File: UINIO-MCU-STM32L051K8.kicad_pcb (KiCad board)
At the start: 2 copper layers, 48.4 x 20.5 mm, 33 parts, among them J1 Conn_01x14_Male, J2 Conn_01x14_Male, J3 Conn_01x04_Male, SW1 SW_Push, SW2 SW_Push, U1 ME6211, U2 W25Q128JVSSIQ, U3 STM32L051K8U6, Y1 Crystal-FC135-32.768

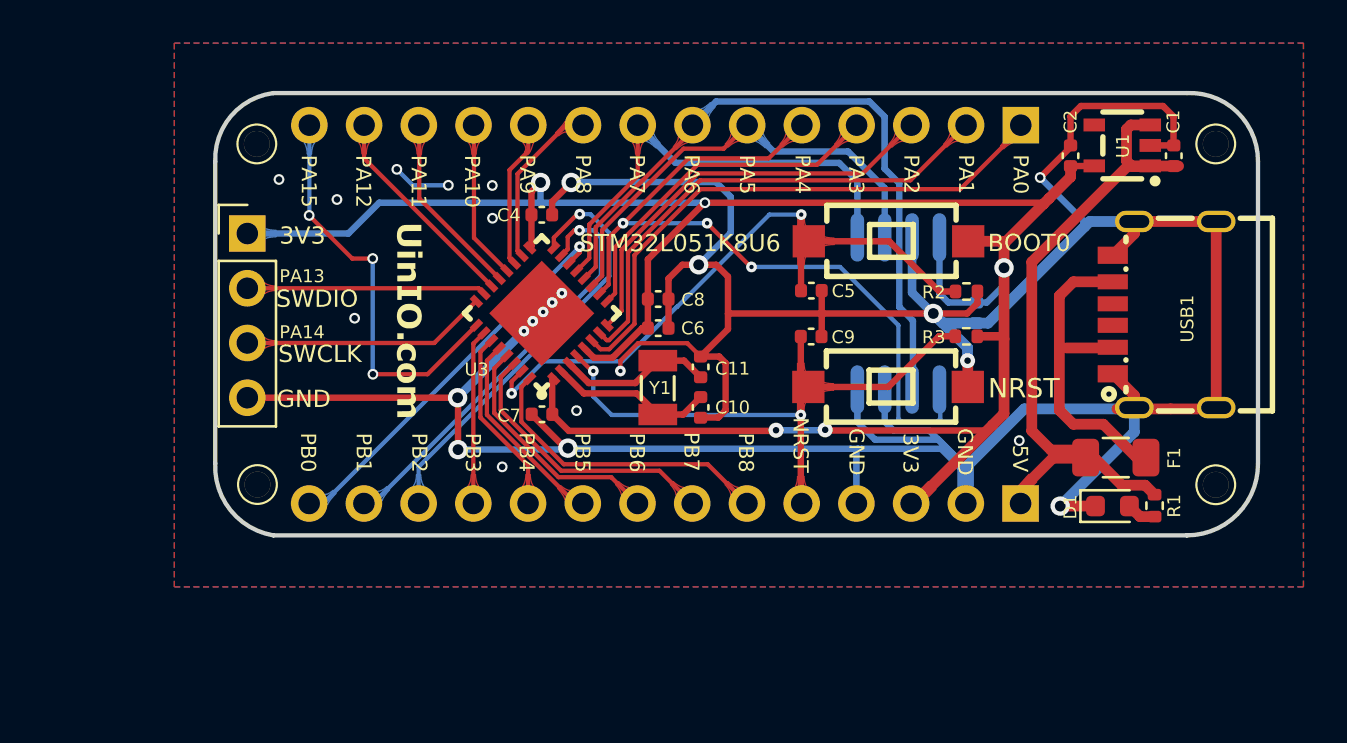
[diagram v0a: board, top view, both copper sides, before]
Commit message: Release UINIO-MCU-STM32L051K8 version 3.2.0.
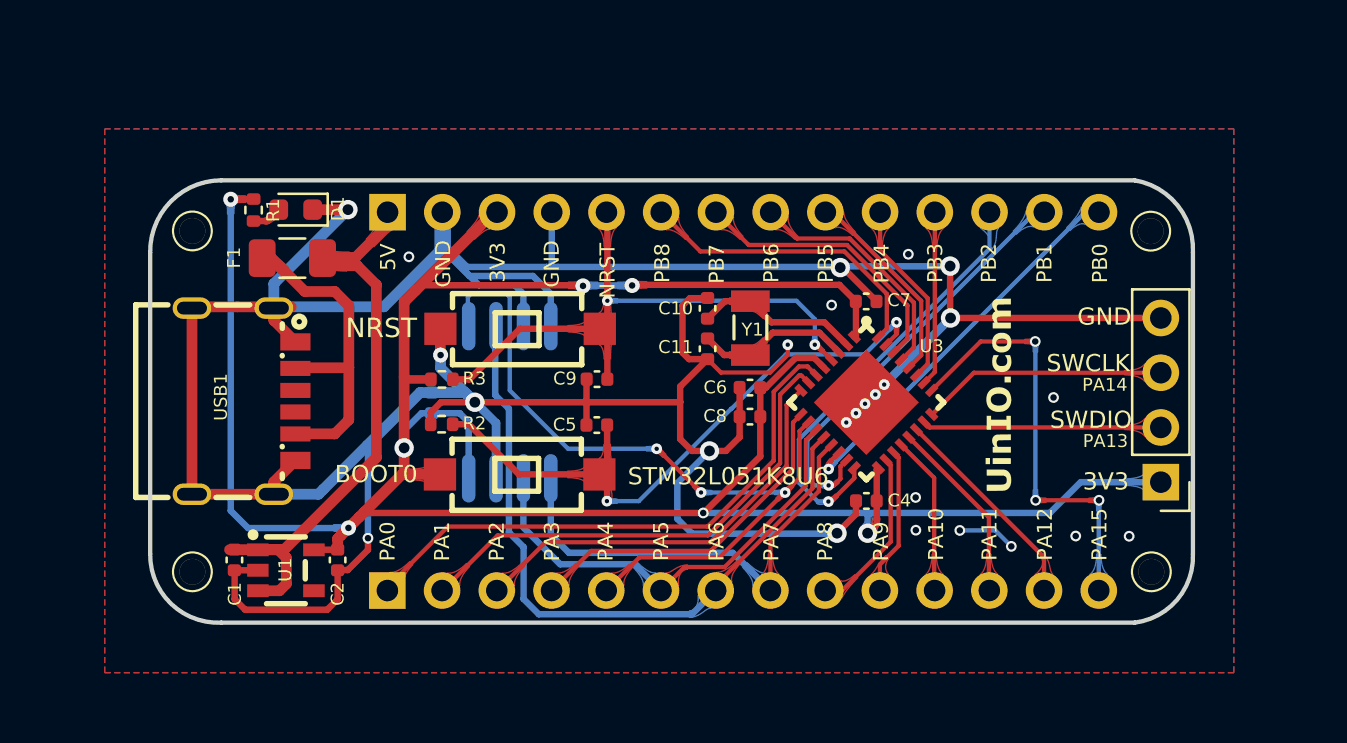
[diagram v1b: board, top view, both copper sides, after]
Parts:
- moved Hole4 51.5 mm to (127.5, 111.7), turned to 180 degrees
- moved Hole3 48.9 mm to (127.5, 95.8), turned to 180 degrees
- moved C1 47.5 mm to (129.5, 111.1), turned to 90 degrees
- moved Hole1 46.0 mm to (172.1, 111.7), turned to 180 degrees
- moved R1 44.0 mm to (130.4, 94.9)
- moved J3 43.9 mm to (172.5, 107.5), turned to 180 degrees
- moved U1 43.5 mm to (131.9, 111.6), turned to 180 degrees
- moved Hole2 43.1 mm to (172.0, 95.9), turned to 180 degrees
- moved USB1 42.9 mm to (129.9, 103.8), turned to -90 degrees
- moved D1 40.3 mm to (132.3, 94.9), turned to 180 degrees
- moved F1 39.3 mm to (132.2, 97.1), turned to 0 degrees
- moved C2 38.8 mm to (134.3, 111.1), turned to 90 degrees
- moved J1 36.5 mm to (136.6, 112.5), turned to -90 degrees
- moved J2 32.3 mm to (136.6, 95.0), turned to -90 degrees
- moved ? 32.0 mm to (135.4, 103.7), turned to -90 degrees
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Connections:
- R1 pad 2: /VDD_5V -> /VDD_3.3V
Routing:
- net /VDD_3.3V: track 104.8 -> 126.1 mm, vias 5 -> 7
- net /VDD_5V: track 31.5 -> 28.0 mm
- net GND: track 186.5 -> 188.0 mm
- net /PA15: track 19.1 -> 20.3 mm
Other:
- outline, holes or cut-outs redrawn
- board text added: "Version 3.2.0"
- board text removed: "Version 3.1.0"

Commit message: Update version.
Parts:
- J1, J2: value Conn_01x14_Male -> Conn_01x14_Pin
- J3: value Conn_01x04_Male -> Conn_01x04_Pin

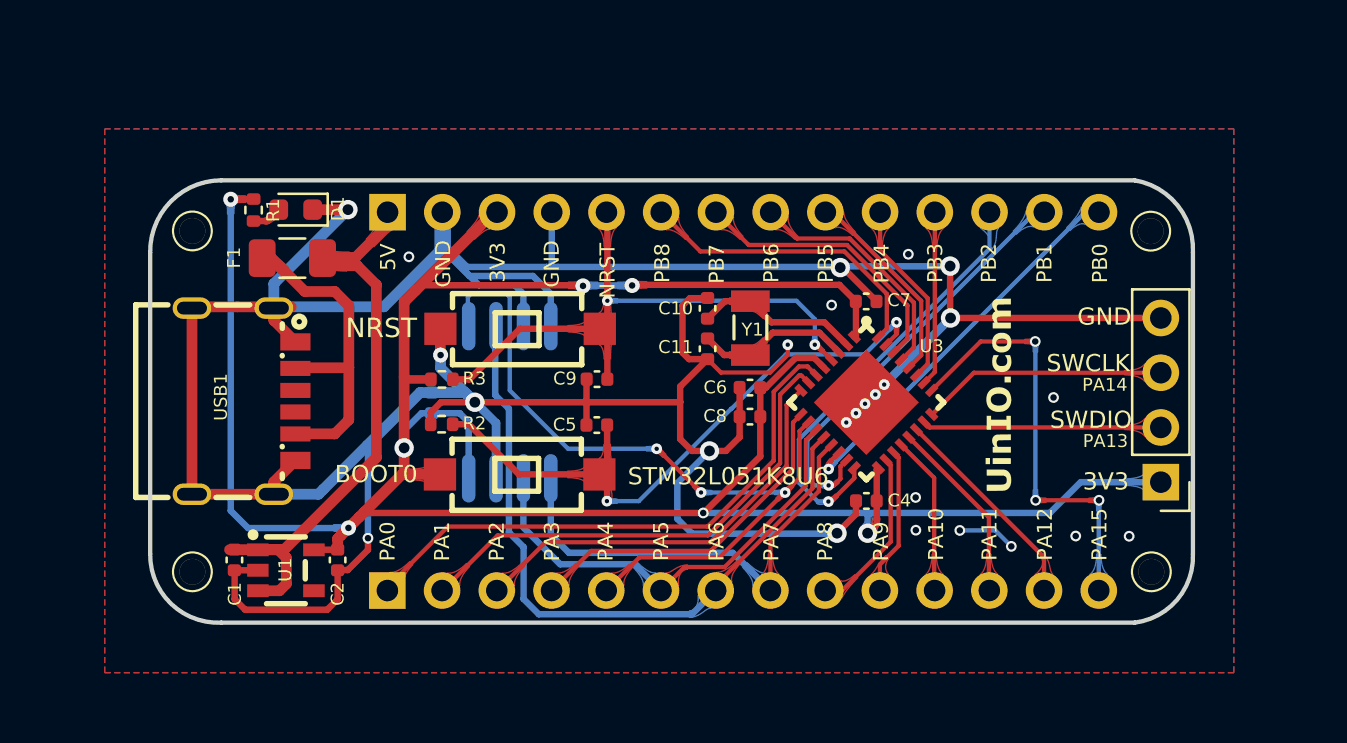
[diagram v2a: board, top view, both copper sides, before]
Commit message: Update PCB.
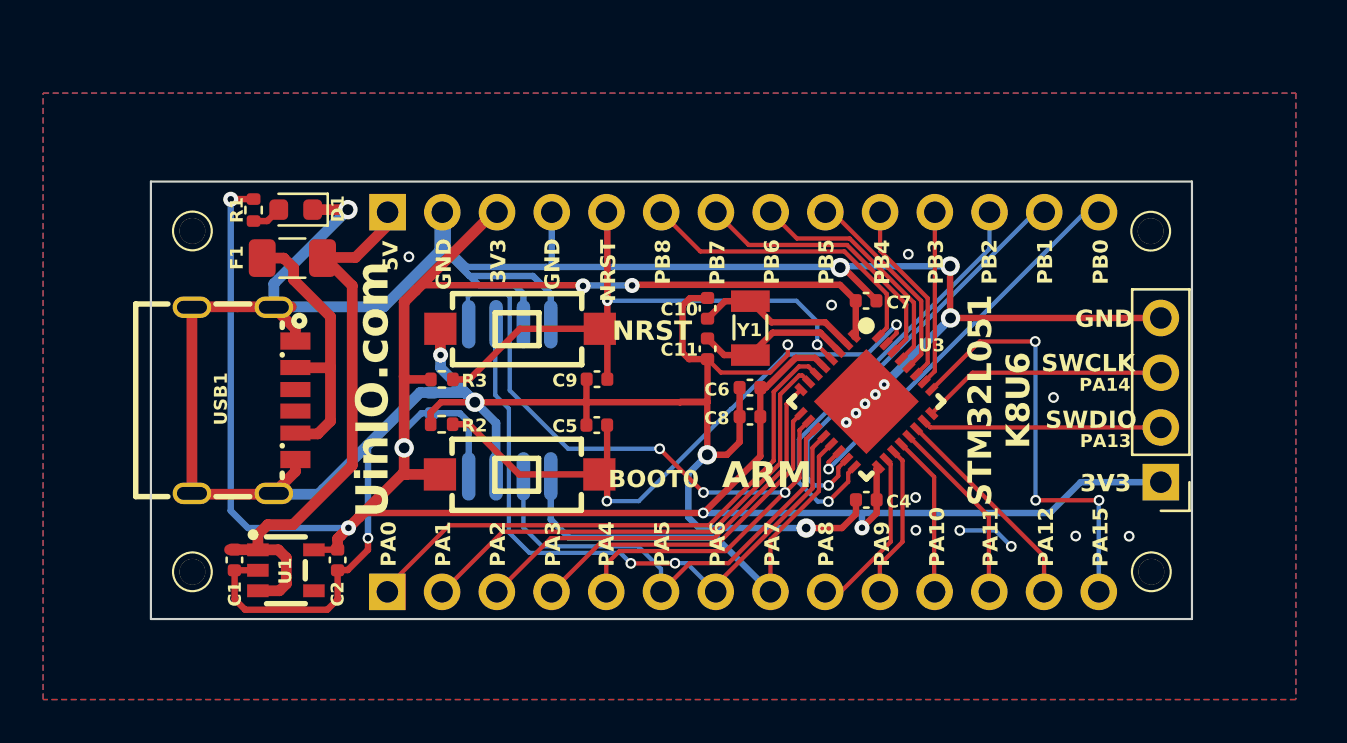
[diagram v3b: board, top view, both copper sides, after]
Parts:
- removed the ? at (164.9, 103.5)
- moved U2 0.09 mm to (142.3, 103.7)
- moved J1 0.06 mm to (136.6, 112.6)
- moved C4 0.05 mm to (158.8, 108.3)
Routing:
- net /PA6/MISO: track 31.8 -> 29.5 mm, vias 0 -> 2
- net Net-(F1-Pad1): track 15.2 -> 13.0 mm
- net /VDD_5V: track 28.0 -> 26.2 mm
- net /PA4/CS: track 36.1 -> 36.9 mm
- net /PA5/SCLK: track 21.4 -> 22.1 mm
- net /PA8: track 7.86 -> 7.20 mm
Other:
- board size 48.4 x 20.5 mm -> 48.3 x 20.3 mm
- board text added: "ARM"
- board text added: "STM32L051 K8U6"
- board text added: "UinIO.com"
- board text added: "Version 3.3.0"
- board text removed: "STM32L051K8U6"
- board text removed: "Version 3.2.0"
